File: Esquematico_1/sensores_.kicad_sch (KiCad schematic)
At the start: 10 parts, among them IC1 MAX-M10M-00B, U1 Gyro, U3 Mag, U4 BMP388

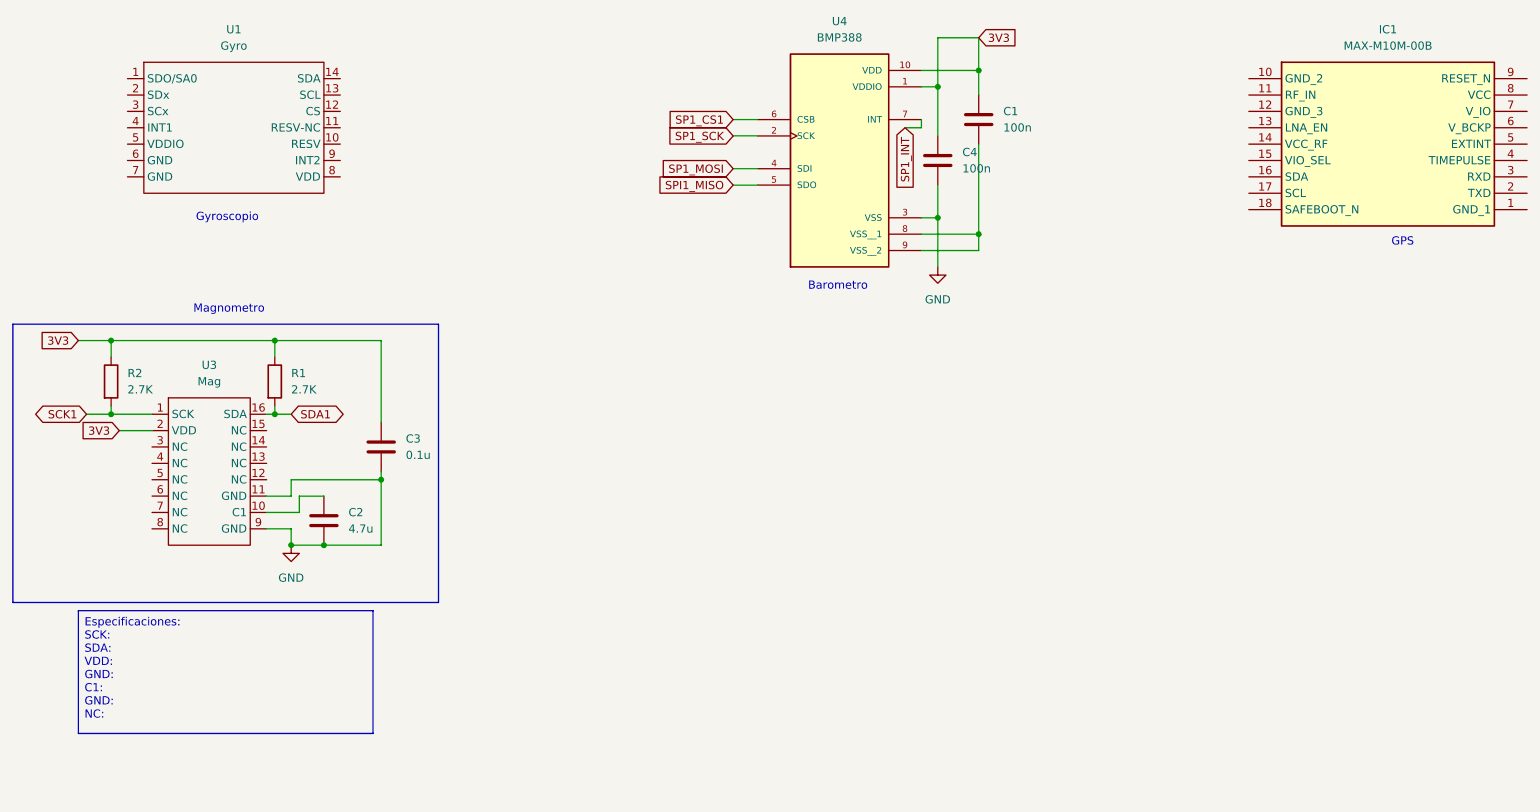
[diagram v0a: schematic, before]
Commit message: Descripcion de esquematicos
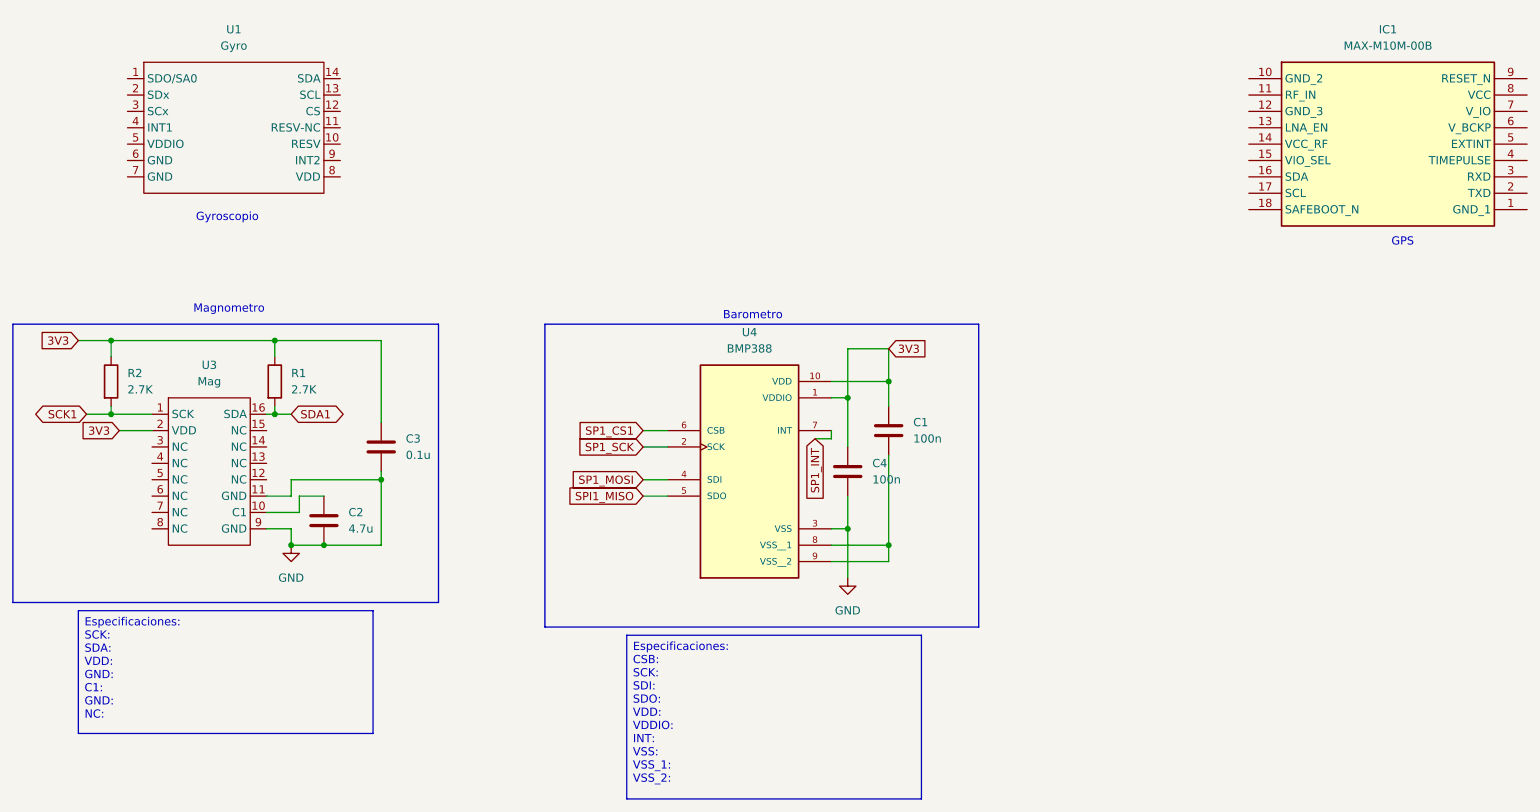
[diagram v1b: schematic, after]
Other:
- moved on the sheet: C1, C4, U4
